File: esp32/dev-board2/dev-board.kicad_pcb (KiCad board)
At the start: 2 copper layers, 57.8 x 31.8 mm, 25 parts, among them J1 USB_B_Micro, J2 Conn_01x18_Male, J3 Conn_01x18_Male, J4 Conn_01x03_Male, Q1 MTB3904-2, U1 AP7361C-33Y5-13, U2 FT231XS, U3 ESP32-WROVER-E

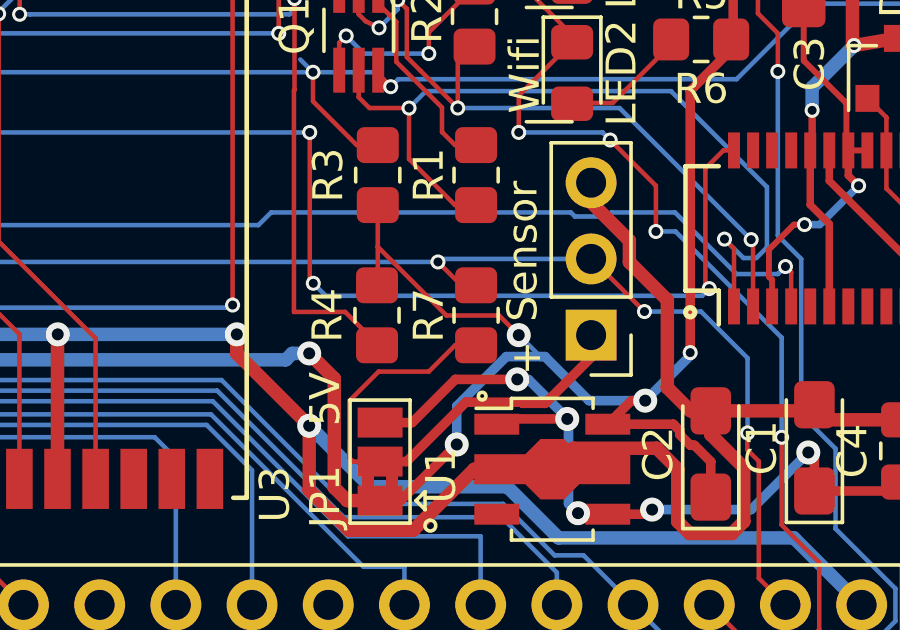
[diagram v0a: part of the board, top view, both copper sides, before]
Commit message: Fixed keywords for PCB
[git-p4: depot-paths = "//depot/nixiestat/": change = 358]
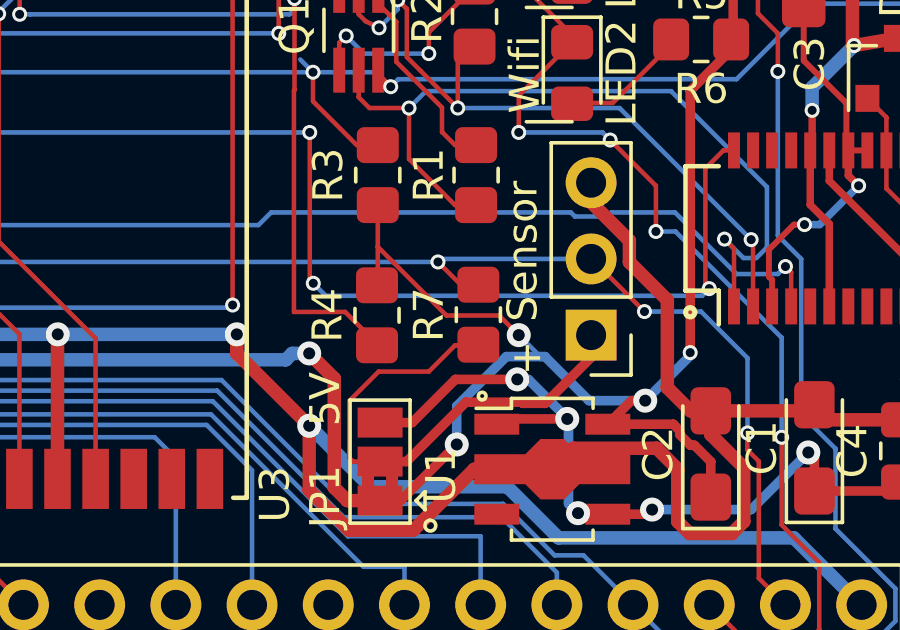
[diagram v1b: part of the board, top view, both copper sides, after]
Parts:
- moved R7 0.08 mm to (142.1, 107.9)
